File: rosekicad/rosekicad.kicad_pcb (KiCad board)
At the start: 4 copper layers, 74 parts, among them J1 Solenoid, J10 Solenoid, J11 Solenoid, J12 Solenoid, J13 UV Lights, J14 LED Lights, J15 DMX Cable, J16 Barrel_Jack_MountingPin, J2 Solenoid, J3 Solenoid, J4 Solenoid, J5 Solenoid, J6 Solenoid, J7 Solenoid, J8 Solenoid, J9 Solenoid, Q1 2N2222, Q10 2N2222, Q11 2N2222, Q12 2N2222, Q13 2N2222, Q14 2N2222, Q15 2N2222, Q2 2N2222, Q3 2N2222, Q4 2N2222, Q5 2N2222, Q6 2N2222, Q7 2N2222, Q8 2N2222, Q9 2N2222, U1 MAX485E

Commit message: mounting holes
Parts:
- added H1: MountingHole, MountingHole:MountingHole_4.5mm_Pad, F.Cu at (276.9, 38.1)
- added H2: MountingHole, MountingHole:MountingHole_4.5mm_Pad, F.Cu at (99.1, 38.1)
- added H3: MountingHole, MountingHole:MountingHole_4.5mm_Pad, F.Cu at (99.1, 190.5)
- added H4: MountingHole, MountingHole:MountingHole_4.5mm_Pad, F.Cu at (276.9, 190.5)
- moved J11 83.8 mm to (140.3, 62.4)
- moved J10 83.7 mm to (125.5, 62.4)
- moved J9 83.7 mm to (110.8, 62.4)
- moved C3 83.6 mm to (175.6, 53.9)
- moved J12 83.6 mm to (154.3, 62.4)
- moved Q12 83.6 mm to (154.6, 76.7)
- moved Q15 83.6 mm to (163.8, 55.2)
- moved R19 83.6 mm to (176.9, 43.8)
- moved R23 83.6 mm to (154.3, 46.4)
- moved R25 83.6 mm to (130.1, 80.2)
- moved R26 83.6 mm to (145.6, 80.2)
- moved R27 83.6 mm to (158.8, 79.7)
- moved A1 83.6 mm to (242.4, 106.3)
- moved C1 83.6 mm to (173.4, 153.3)
- moved C2 83.6 mm to (173.7, 104.0)
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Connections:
- A1 pad 5: Net-(A1-+5V) -> +5V
- C4 pad 1: Net-(A1-+5V) -> +5V
- U1 pad 1: unconnected-(U1-RO-Pad1) -> Net-(A1-D1/TX)
- U1 pad 4: Net-(A1-D1/TX) -> unconnected-(U1-DI-Pad4)
- U1 pad 8: Net-(A1-+5V) -> +5V
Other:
- board outline added: 203.2 x 177.8 mm

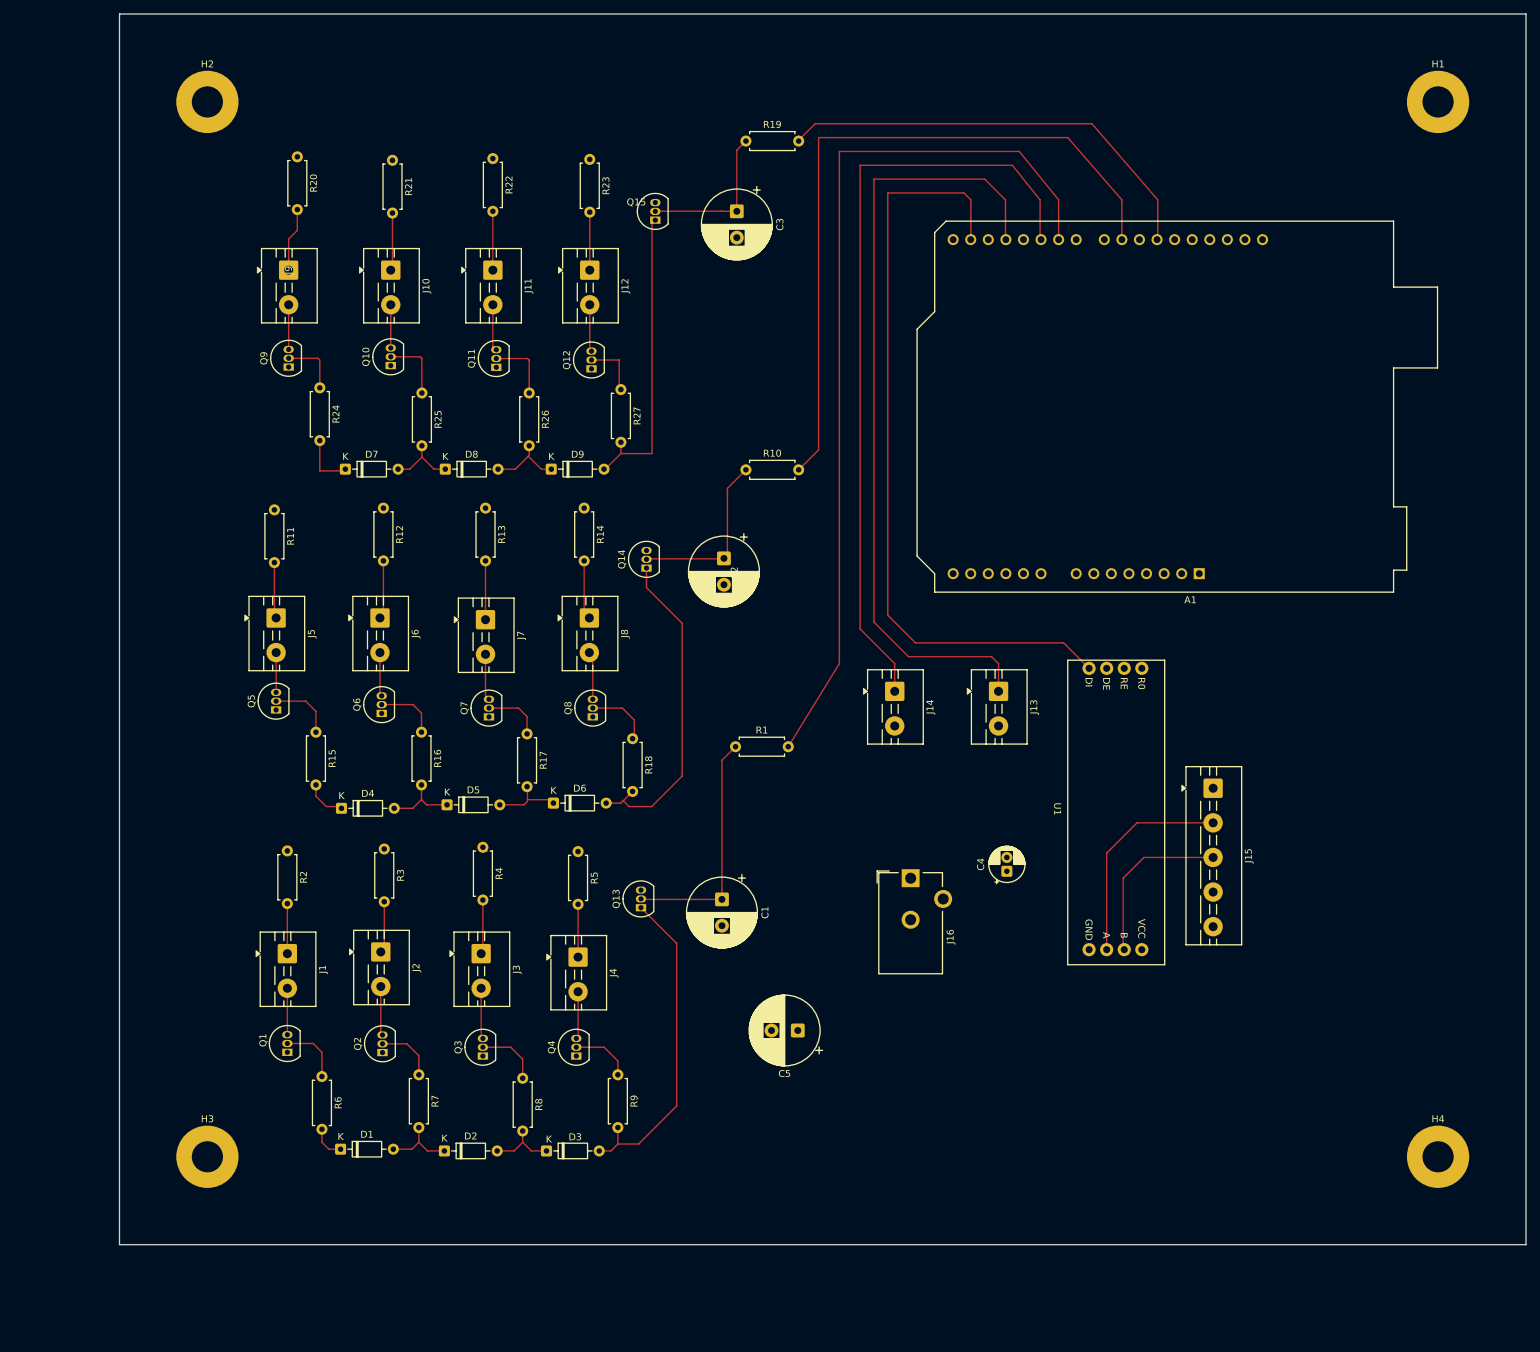
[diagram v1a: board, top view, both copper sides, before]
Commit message: finalized pcb main
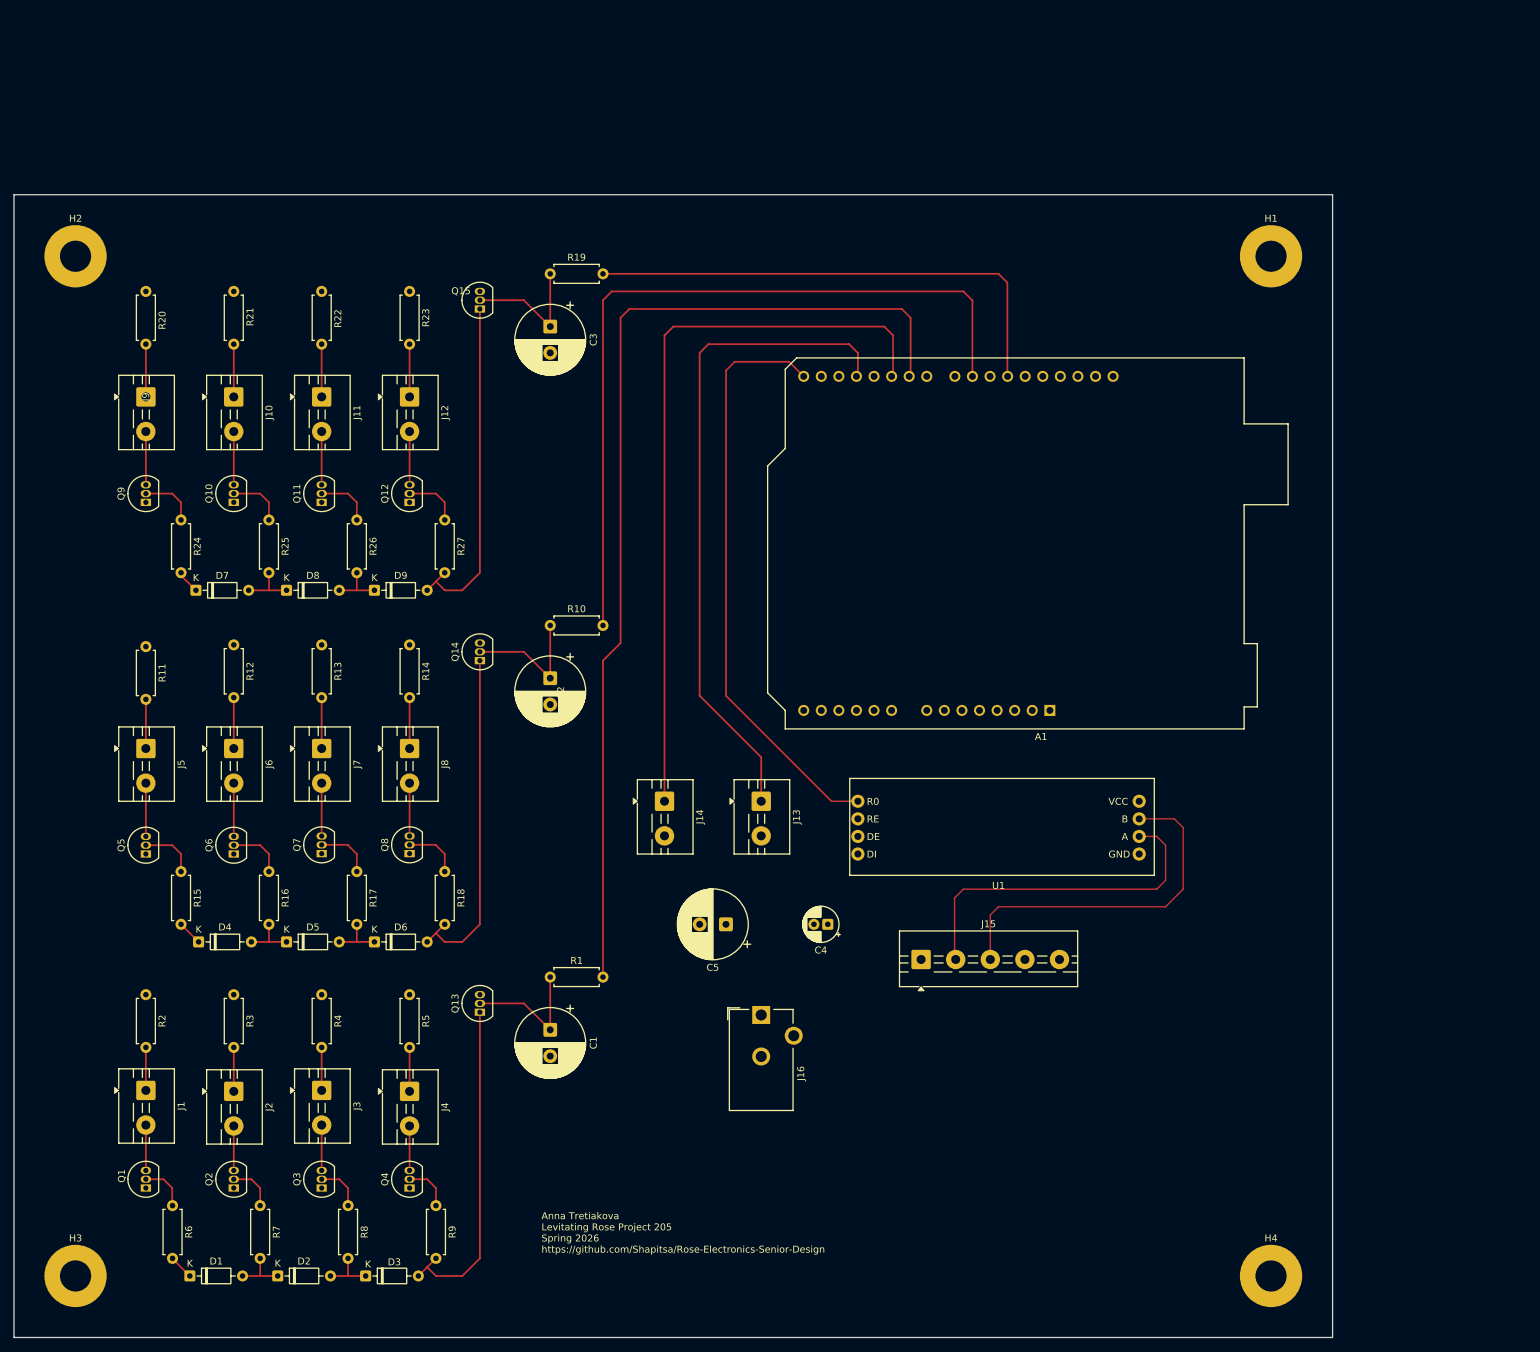
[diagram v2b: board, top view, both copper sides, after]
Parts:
- moved J15 48.9 mm to (202.2, 162.0), turned to 0 degrees
- moved R1 42.7 mm to (148.6, 164.5)
- moved J13 37.8 mm to (179.1, 139.1)
- moved J14 36.9 mm to (165.1, 139.1)
- moved R10 36.1 mm to (148.6, 113.7)
- moved R19 34.2 mm to (148.6, 62.9)
- moved R18 33.2 mm to (133.3, 149.3)
- moved Q8 33.0 mm to (128.3, 146.7)
- moved H1 32.9 mm to (252.7, 60.4)
- moved D6 32.7 mm to (123.2, 159.5)
- moved Q12 32.6 mm to (128.3, 96.0)
- moved R9 32.4 mm to (132.1, 197.6)
- moved R23 32.3 mm to (128.3, 65.5)
- moved J8 32.1 mm to (128.3, 131.5)
- moved R14 32.0 mm to (128.3, 116.5)
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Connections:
- A1 pad 15: unconnected-(A1-D0/RX-Pad15) -> Net-(A1-D0/RX)
- A1 pad 16: Net-(A1-D1/TX) -> unconnected-(A1-D1/TX-Pad16)
- U1 pad 1: Net-(A1-D1/TX) -> Net-(A1-D0/RX)
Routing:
- net Net-(A1-D1/TX): track 111.4 -> 0.00 mm
- net Net-(A1-D0/RX): track 0.00 -> 85.0 mm
- net Net-(J15-Pin_3): track 24.6 -> 51.6 mm
- net Net-(A1-D6): track 128.8 -> 147.8 mm
- net Net-(J15-Pin_2): track 31.1 -> 49.9 mm
- net Net-(A1-D3): track 114.5 -> 95.8 mm
- net Net-(Q13-B): track 34.6 -> 19.4 mm
- net Net-(A1-D9): track 102.9 -> 112.4 mm
- net Net-(A1-D11): track 63.8 -> 72.5 mm
- net Net-(D9-A): track 43.2 -> 49.6 mm
- net Net-(Q14-B): track 25.2 -> 19.4 mm
- net Net-(A1-D5): track 112.3 -> 107.4 mm
- net Net-(D7-K): track 7.86 -> 3.43 mm
- net +5V: track 4.21 -> 0.00 mm
- net Net-(D8-A): track 11.0 -> 7.62 mm
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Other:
- board size 203.2 x 177.8 mm -> 190.5 x 165.1 mm
- board text added: "Anna Tretiakova Levitating Rose Project 205 Spring 2026 https://github.com/Shapitsa/Rose-Electronics-Senior-Design"
